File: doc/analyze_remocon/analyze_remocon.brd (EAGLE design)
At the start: 58.1 x 27.9 mm, 20 parts, among them IC3 PIC18F2550_28DIP, Q2 BUZ11BV, X1 MINI-USB-UX60-MB-5S8

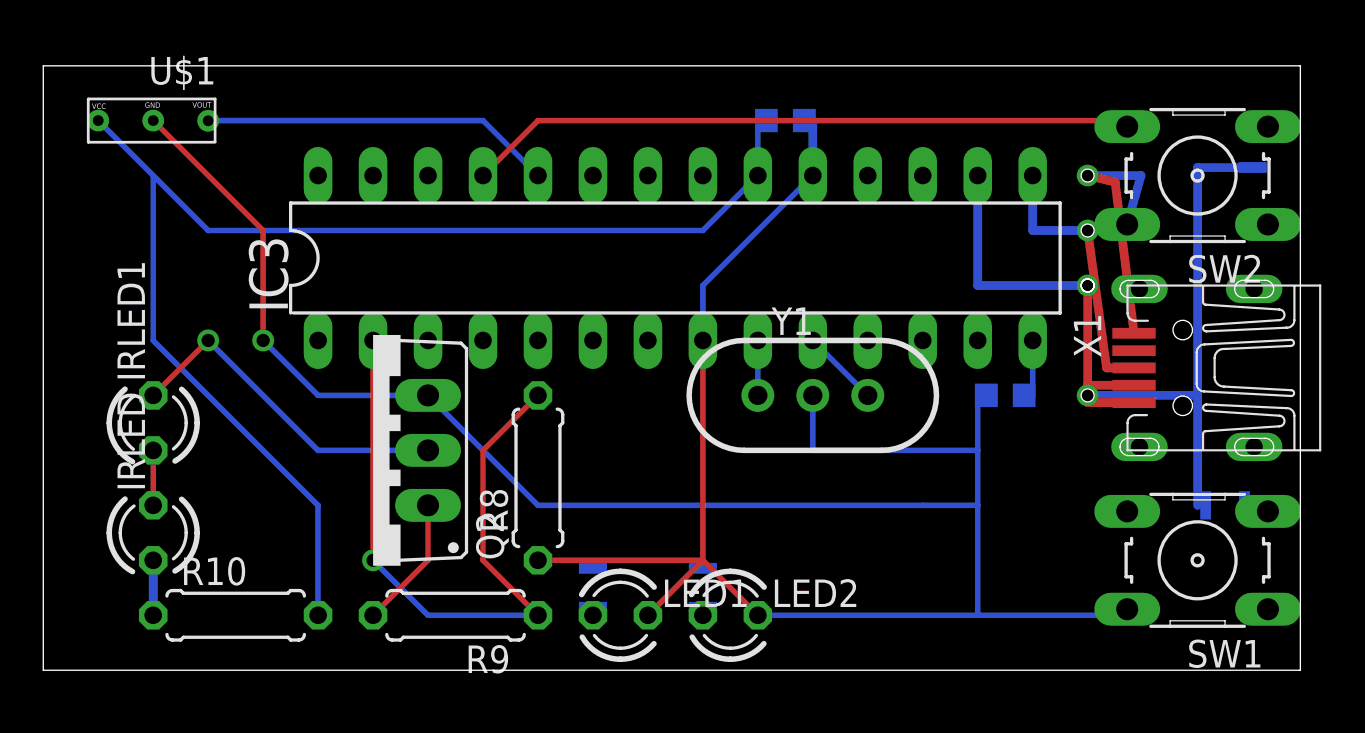
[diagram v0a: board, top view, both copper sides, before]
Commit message: update circuit diagram documents
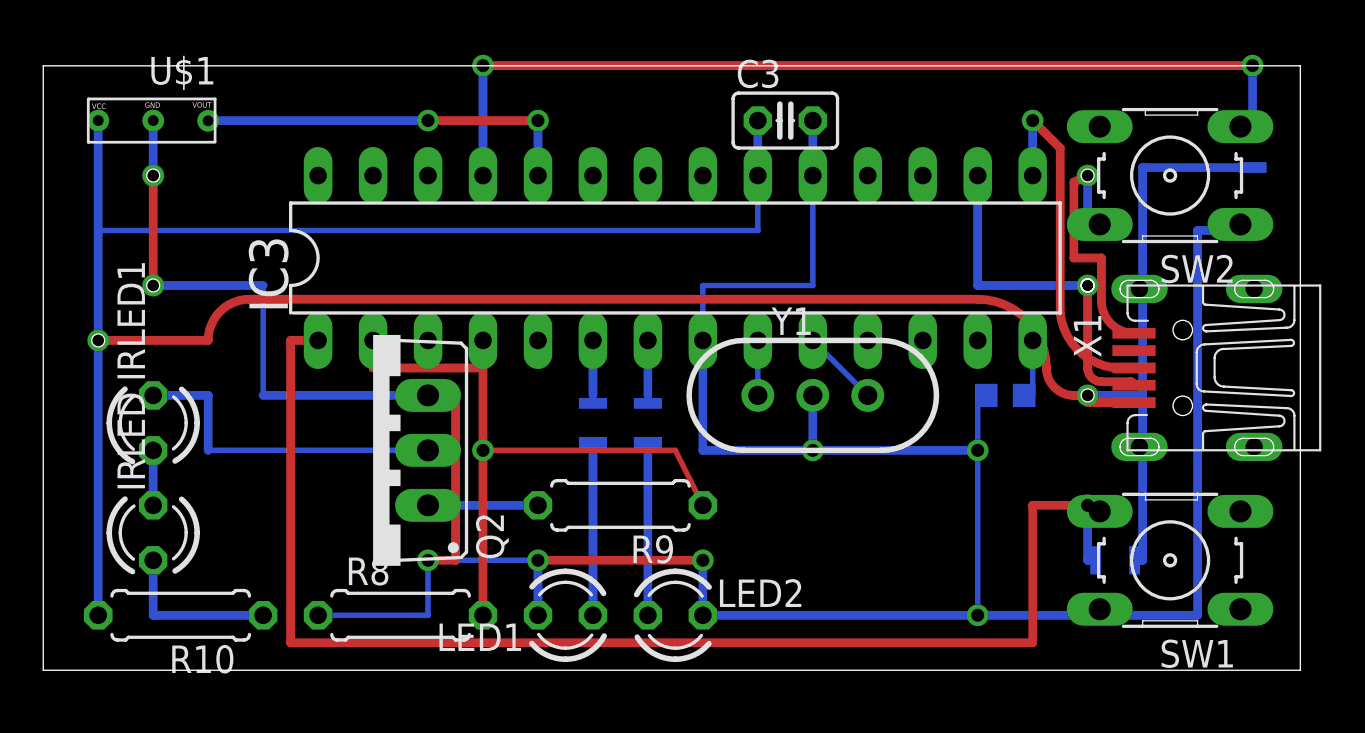
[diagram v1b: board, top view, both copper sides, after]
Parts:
- removed C1: (no value), rcl:C0603K
- added C3: (no value), rcl:C025-025X050
- moved R9 9.16 mm to (26.7, 7.62)
- moved R8 8.98 mm to (16.5, 2.54), turned to 0 degrees
- moved R7 8.03 mm to (27.9, 11.4)
- moved R6 7.62 mm to (25.4, 11.4)
- moved R1 5.68 mm to (49.5, 5.08), turned to 180 degrees
- moved LED1 2.54 mm to (24.1, 2.54), turned to 180 degrees
- moved R10 2.54 mm to (6.35, 2.54), turned to 180 degrees
- moved LED2 2.54 mm to (29.2, 2.54)
- moved SW1 1.27 mm to (52.1, 5.08)
- moved SW2 1.27 mm to (52.1, 22.9)
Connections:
- removed net N$3: R1.1, SW1.3
- removed net N$5: R2.1, SW2.3
- removed net N$6: IC3.25, SW2.4
- new net N$7: IC3.25, R2.1, SW2.3
- net BLOCK: now also C3.1; no longer C1.1
- net GND: now also C3.2, SW2.1; no longer C1.2
- net N$4: now also R1.1
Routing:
- net N$4: track 0.00 -> 62.0 mm, vias 0 -> 1
- net BLOCK: track 85.8 -> 135.4 mm, vias 1 -> 2
- net N$7: track 0.00 -> 43.8 mm, vias 0 -> 2
- net N$6: track 32.3 -> 0.00 mm
- net GND: track 138.5 -> 164.2 mm, vias 2 -> 9
- net N$13: track 0.00 -> 7.62 mm
- net N$11: track 0.00 -> 7.62 mm
- net N$15: track 2.54 -> 7.62 mm
- net N$2: track 12.8 -> 16.0 mm
- net N$9: track 0.00 -> 2.54 mm
- net N$12: track 0.00 -> 2.54 mm
- net N$14: track 31.1 -> 29.5 mm
- net N$19: track 16.3 -> 17.8 mm, vias 0 -> 2
- net N$18: track 6.13 -> 5.08 mm
- net N$17: track 15.9 -> 15.2 mm, vias 1 -> 0
